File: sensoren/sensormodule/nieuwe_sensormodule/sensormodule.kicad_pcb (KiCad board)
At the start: 2 copper layers, 12 parts, among them J1 Screw_Terminal_01x05, U1 TCRT5000, U2 TCRT5000, U3 TCRT5000

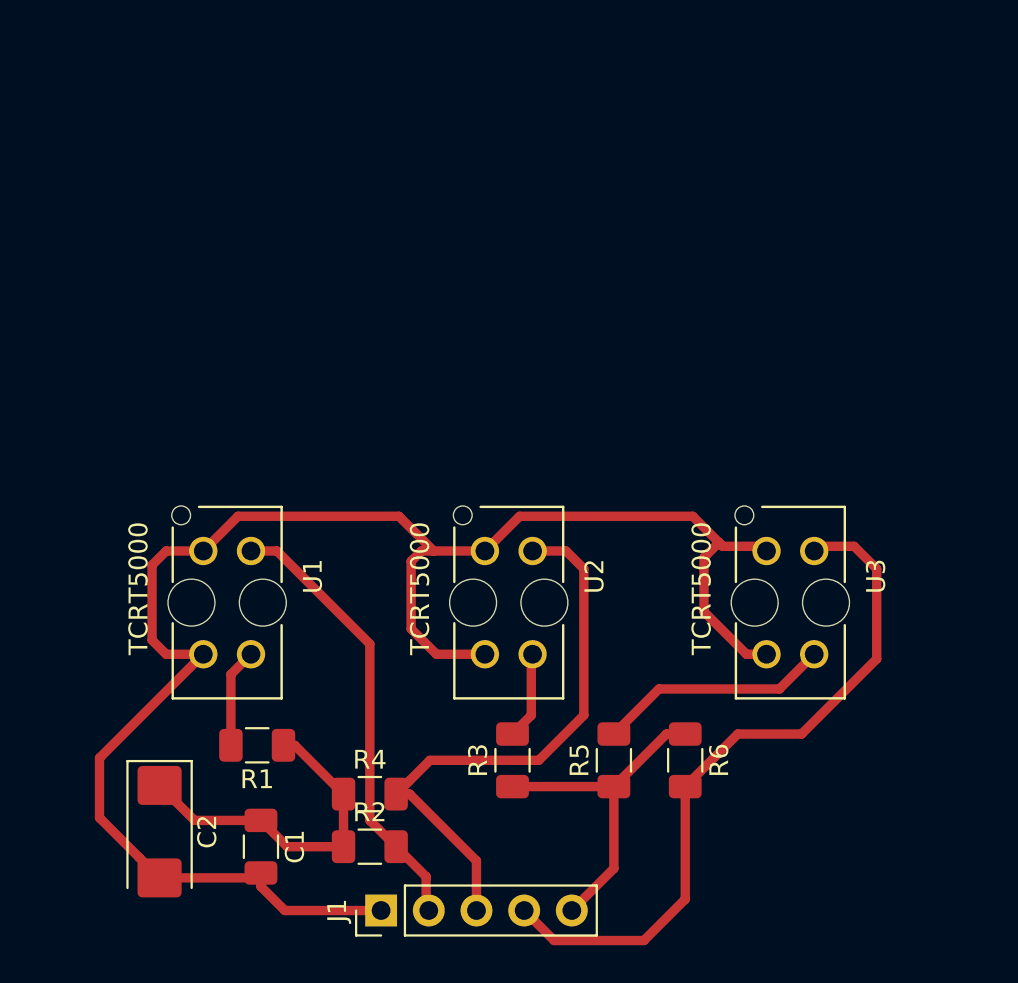
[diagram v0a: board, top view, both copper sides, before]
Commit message: routing nieuwe sens
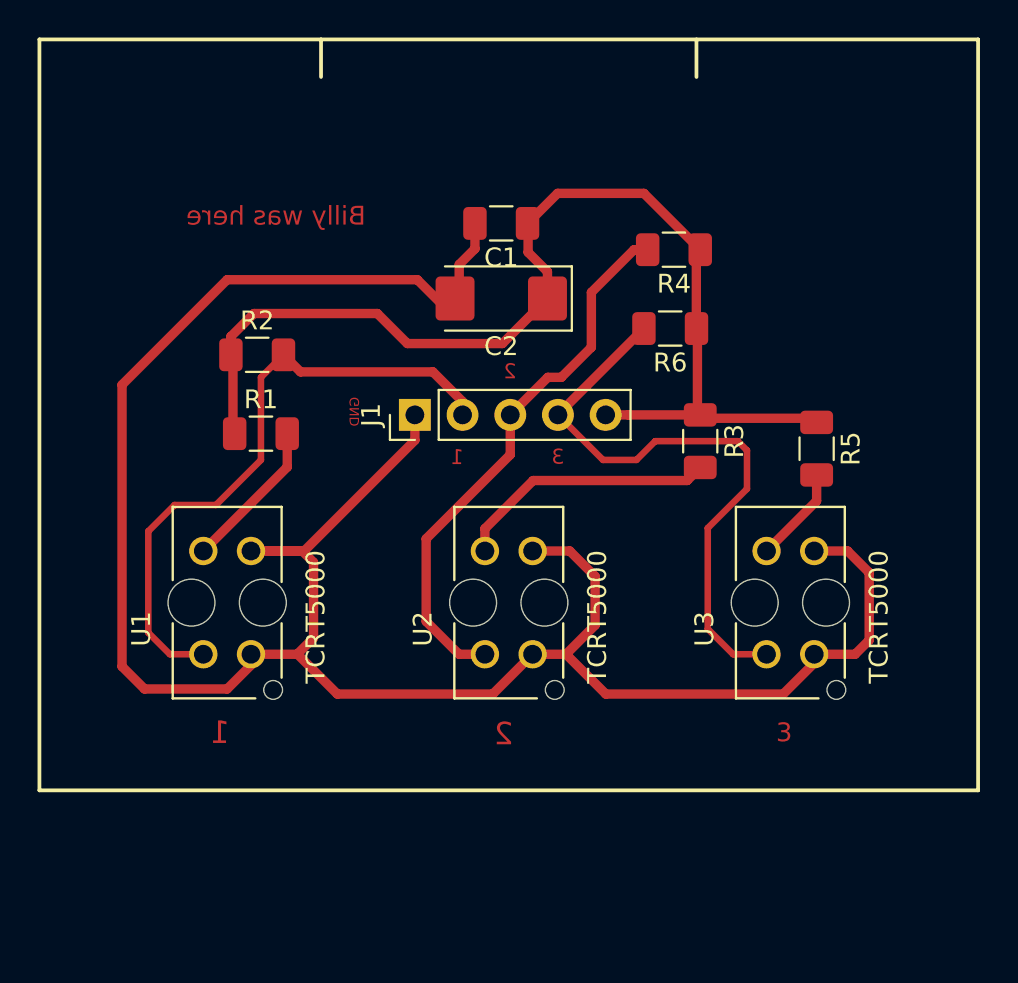
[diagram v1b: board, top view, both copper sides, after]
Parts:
- moved C1 35.6 mm to (119.6, 39.8), turned to 180 degrees
- moved C2 33.7 mm to (119.6, 43.8), turned to 180 degrees
- moved R4 33.2 mm to (128.8, 41.2), turned to 180 degrees
- moved R2 26.9 mm to (106.6, 46.8)
- moved J1 26.5 mm to (115.0, 50.0)
- moved R6 23.0 mm to (128.6, 45.4), turned to 180 degrees
- moved R5 19.8 mm to (136.4, 51.8), turned to 270 degrees
- moved R3 19.7 mm to (130.2, 51.4), turned to 270 degrees
- moved R1 16.6 mm to (106.8, 51.0), turned to 0 degrees
- turned U1 to 90 degrees
- turned U2 to 90 degrees
- turned U3 to 90 degrees
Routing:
- net GND: track 89.9 -> 122.9 mm
- net +5V: track 36.1 -> 60.2 mm
- net Net-(J1-Pad2): track 23.9 -> 33.8 mm
- net Net-(R3-Pad2): track 4.69 -> 14.0 mm
- net Net-(R5-Pad2): track 12.4 -> 5.16 mm
- net Net-(J1-Pad4): track 37.9 -> 32.2 mm
- net Net-(R1-Pad2): track 5.29 -> 8.10 mm
- net Net-(J1-Pad3): track 31.1 -> 29.4 mm
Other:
- board text added: "1"
- board text added: "2"
- board text added: "3"
- board text added: "Billy was here"
- board text added: "GND"
